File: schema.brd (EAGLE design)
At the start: 50.5 x 53.3 mm, 21 parts, among them T1 2N2222, U1 ESP12E, U2 LM2596-L, X1 +5V

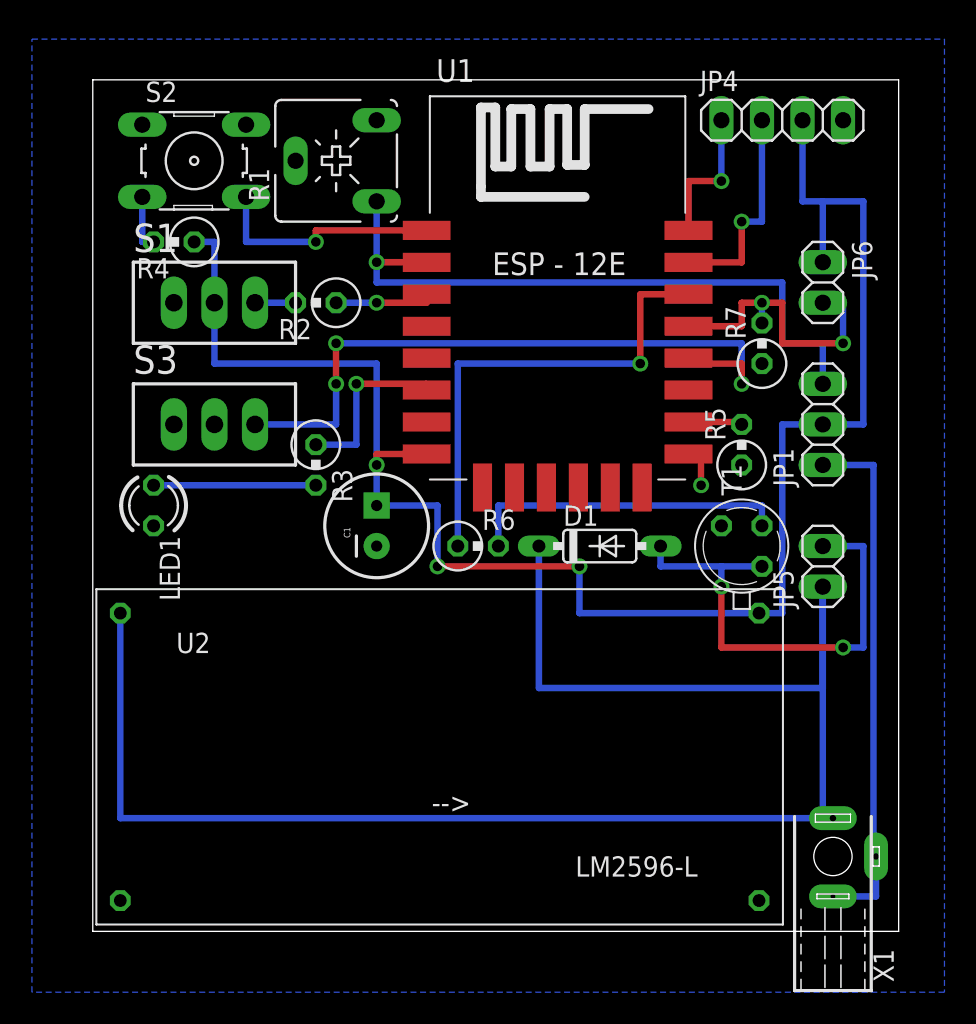
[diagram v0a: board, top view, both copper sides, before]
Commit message: new Eagle version
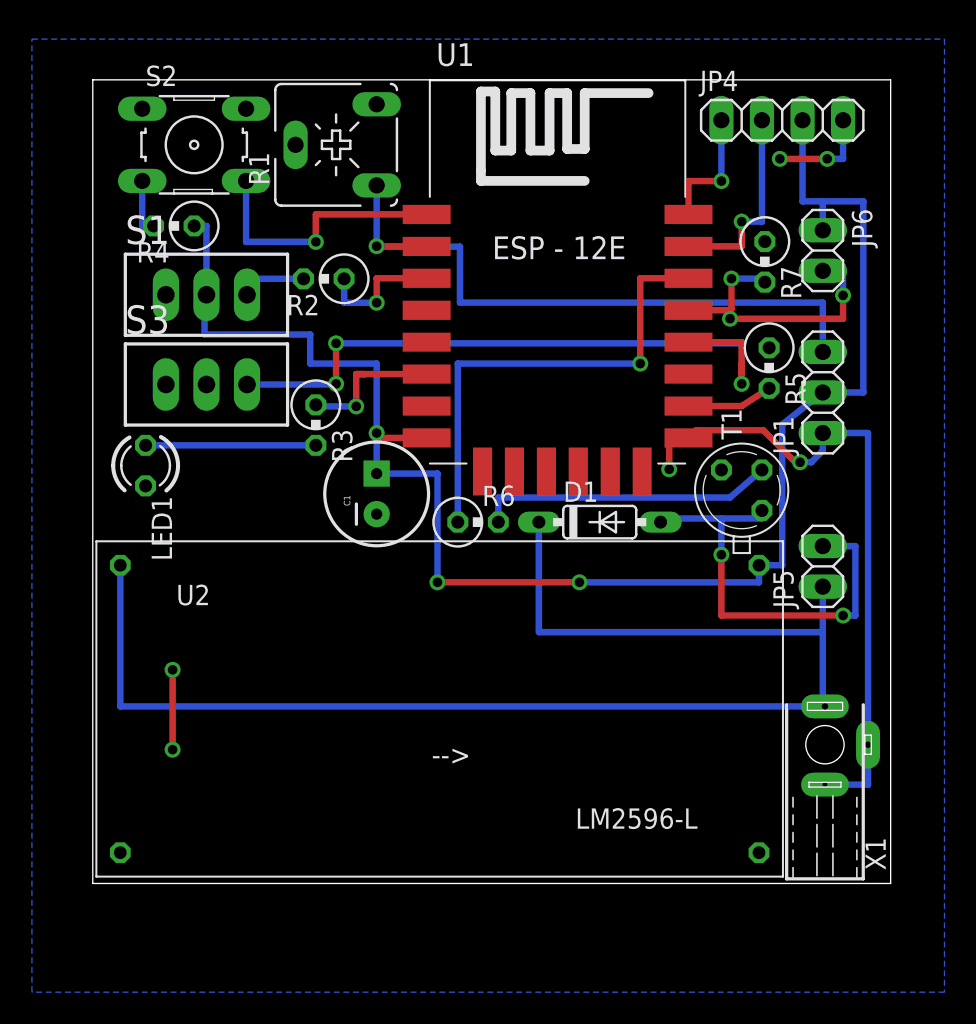
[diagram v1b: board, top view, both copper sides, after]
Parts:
- moved X1 7.02 mm to (45.9, 15.9)
- moved R7 5.10 mm to (42.1, 49.5), turned to 270 degrees
- moved R5 5.10 mm to (42.4, 42.9), turned to 270 degrees
- moved T1 3.50 mm to (40.6, 35.2)
- moved U2 3.00 mm to (22.2, 22.1)
- moved LED1 2.55 mm to (3.31, 36.8)
- moved S3 2.55 mm to (7.12, 41.9)
- moved R3 2.50 mm to (14.0, 39.3)
- moved C1 2.00 mm to (17.8, 35.0)
- moved JP1 2.00 mm to (45.7, 41.4)
- moved JP6 2.00 mm to (45.7, 50.3)
- moved R2 1.58 mm to (14.5, 48.5)
- moved D1 1.50 mm to (31.8, 33.2)
- moved R6 1.50 mm to (24.1, 33.2)
- moved R1 1.00 mm to (15.2, 56.9)
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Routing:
- net +5V: track 106.9 -> 86.4 mm
- net GND: track 35.8 -> 53.0 mm, vias 1 -> 6
- net +3V3: track 107.5 -> 101.2 mm
- net PUMP_GND: track 30.5 -> 27.9 mm
- net CH_PD_S: track 2.54 -> 4.54 mm
- net CH_PD: track 6.20 -> 8.20 mm
- net RST: track 14.8 -> 16.8 mm
- net GPIO15: track 3.48 -> 5.38 mm
- net GPIO5_T: track 20.3 -> 18.7 mm
- net GPIO12: track 11.1 -> 9.56 mm
- net TX: track 8.96 -> 7.96 mm
- net RX: track 13.5 -> 12.5 mm
- net ADC: track 42.5 -> 41.5 mm
- net GPIO5: track 30.2 -> 29.7 mm
- net GPIO12D: track 10.2 -> 10.7 mm
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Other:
- board size 50.5 x 53.3 mm -> 50 x 50.3 mm
